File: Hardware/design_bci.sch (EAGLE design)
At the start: 13 parts, among them IC1 AD623N

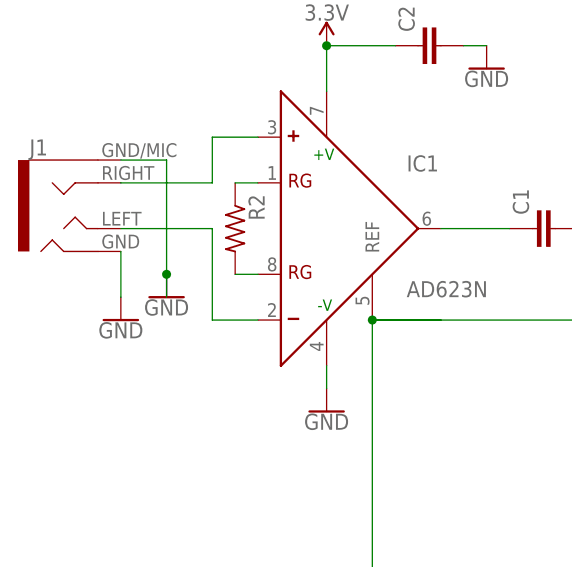
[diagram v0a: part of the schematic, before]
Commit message: made unnoticeable change
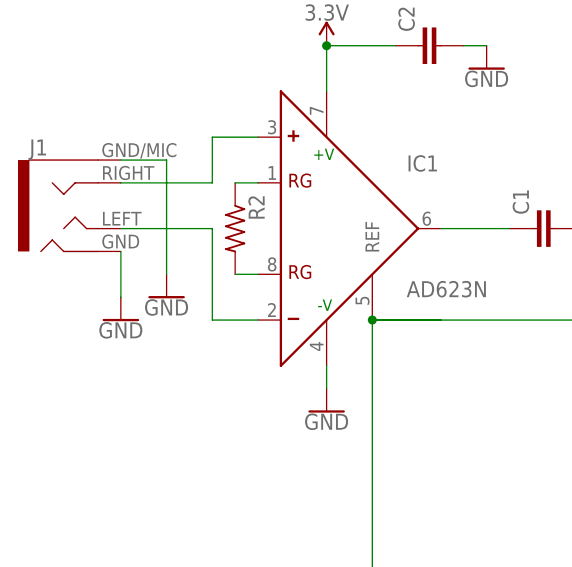
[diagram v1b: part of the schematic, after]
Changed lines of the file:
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@@
-</segment>
-<segment>
-<pinref part="J1" gate="G$1" pin="SLEEVE"/>
-<wire x1="-2.54" y1="93.98" x2="2.54" y2="93.98" width="0.1524" layer="91"/>
-<wire x1="2.54" y1="93.98" x2="2.54" y2="81.28" width="0.1524" layer="91"/>
-<pinref part="GND7" gate="G$1" pin="GND"/>
-<wire x1="2.54" y1="81.28" x2="2.54" y2="78.74" width="0.1524" layer="91"/>
-<junction x="2.54" y="81.28"/>
 </segment>
 <segment>
@@
 <junction x="106.68" y="60.96"/>
 </segment>
+<segment>
+<pinref part="J1" gate="G$1" pin="SLEEVE"/>
+<wire x1="-2.54" y1="93.98" x2="2.54" y2="93.98" width="0.1524" layer="91"/>
+<pinref part="GND7" gate="G$1" pin="GND"/>
+<wire x1="2.54" y1="93.98" x2="2.54" y2="81.28" width="0.1524" layer="91"/>
+</segment>
 </net>
